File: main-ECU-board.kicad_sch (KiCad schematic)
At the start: 0 parts

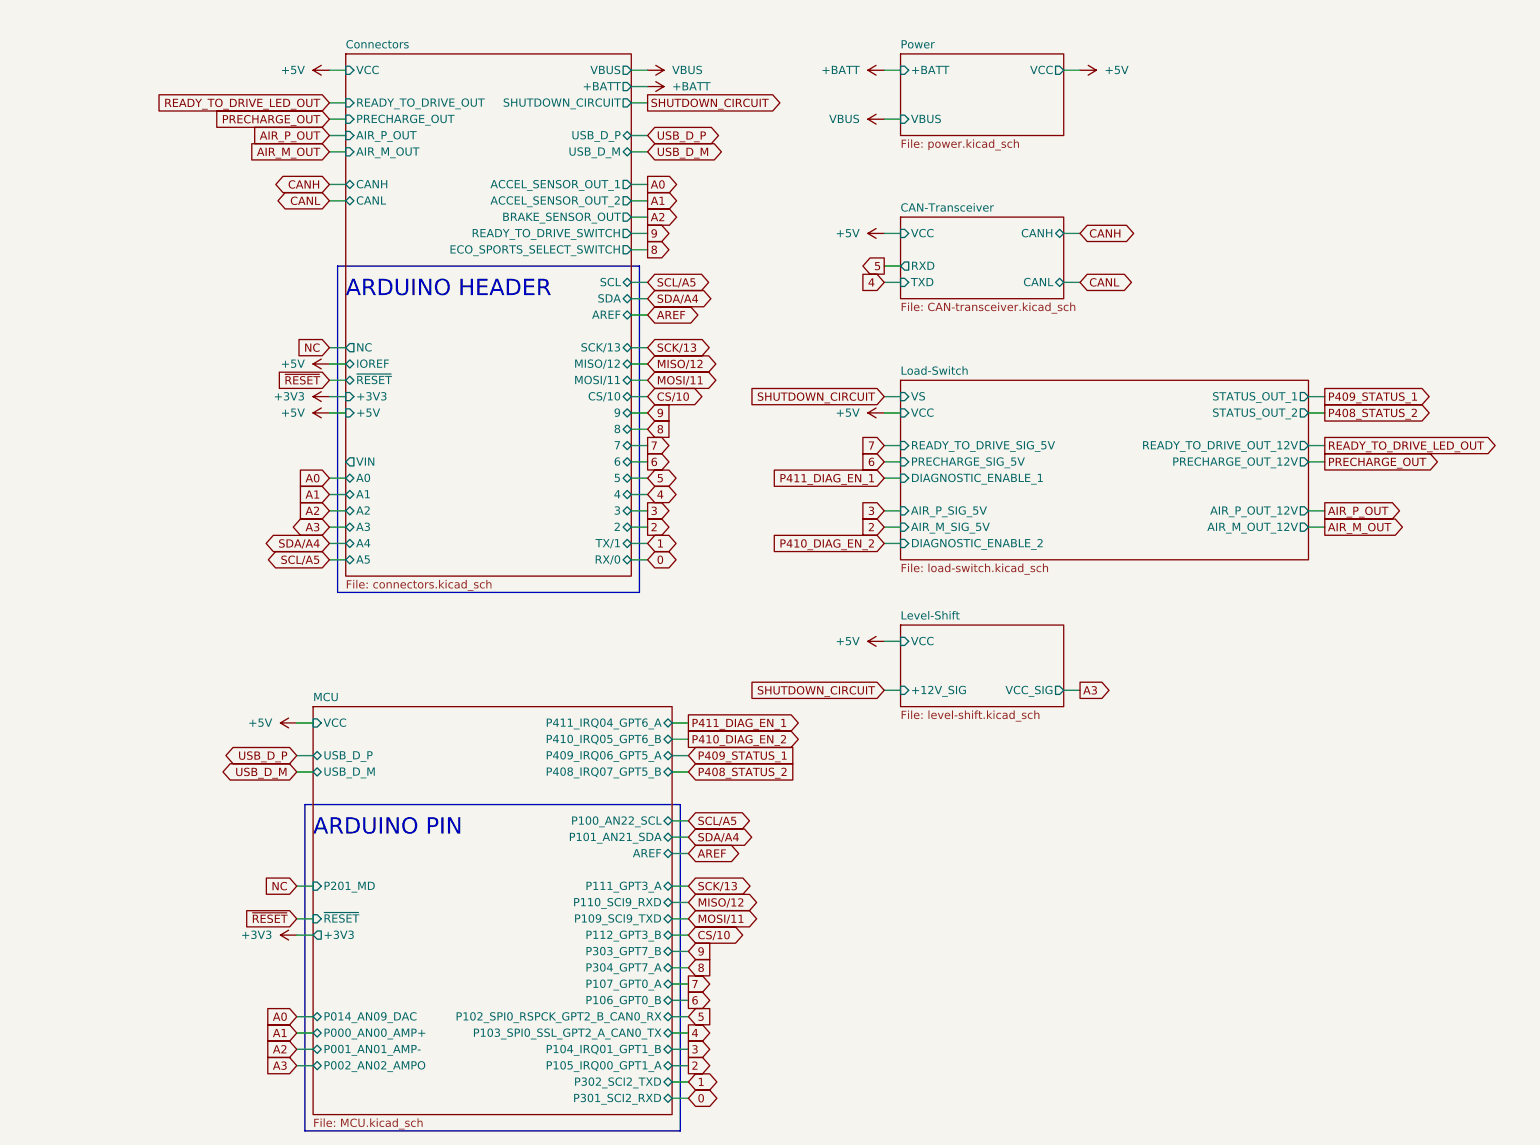
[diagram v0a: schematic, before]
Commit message: modify, add parts
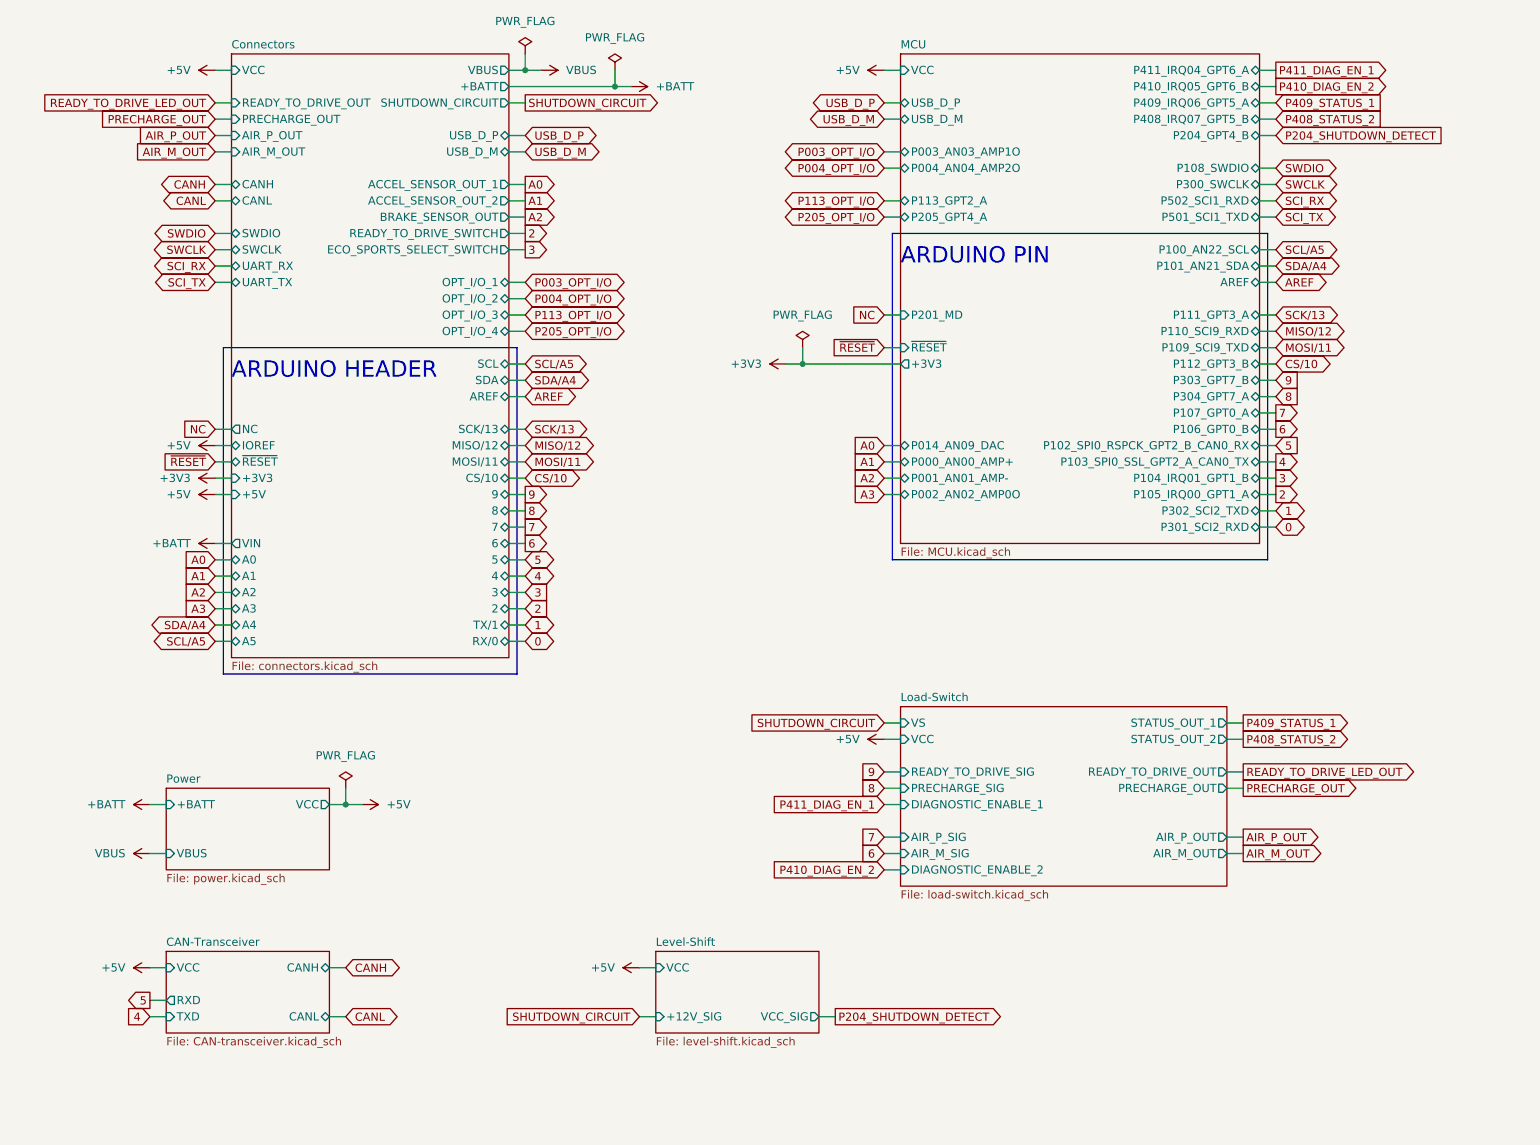
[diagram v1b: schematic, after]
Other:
- sheet Connectors ports: added OPT_I/O_1, OPT_I/O_2, OPT_I/O_3, OPT_I/O_4, SWCLK, SWDIO, UART_RX, UART_TX; removed none
- sheet Load-Switch ports: added AIR_M_OUT, AIR_M_SIG, AIR_P_OUT, AIR_P_SIG, PRECHARGE_OUT, PRECHARGE_SIG, READY_TO_DRIVE_OUT, READY_TO_DRIVE_SIG; removed AIR_M_OUT_12V, AIR_M_SIG_5V, AIR_P_OUT_12V, AIR_P_SIG_5V, PRECHARGE_OUT_12V, PRECHARGE_SIG_5V, READY_TO_DRIVE_OUT_12V, READY_TO_DRIVE_SIG_5V
- sheet MCU ports: added P002_AN02_AMP0O, P003_AN03_AMP1O, P004_AN04_AMP2O, P108_SWDIO, P113_GPT2_A, P204_GPT4_B, P205_GPT4_A, P300_SWCLK, P501_SCI1_TXD, P502_SCI1_RXD; removed P002_AN02_AMPO
